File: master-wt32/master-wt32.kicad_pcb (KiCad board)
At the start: 2 copper layers, 64.6 x 72.4 mm, 24 parts, among them J1 Screw_Terminal_01x04, J2 Screw_Terminal_01x03, J3 Conn_01x06_Female, J4 Conn_01x06_Female, SW1 SW_DIP_x02, U1 MINI360, U2 PC817, U3 WT32-ETH0-Board, U4 MINI360

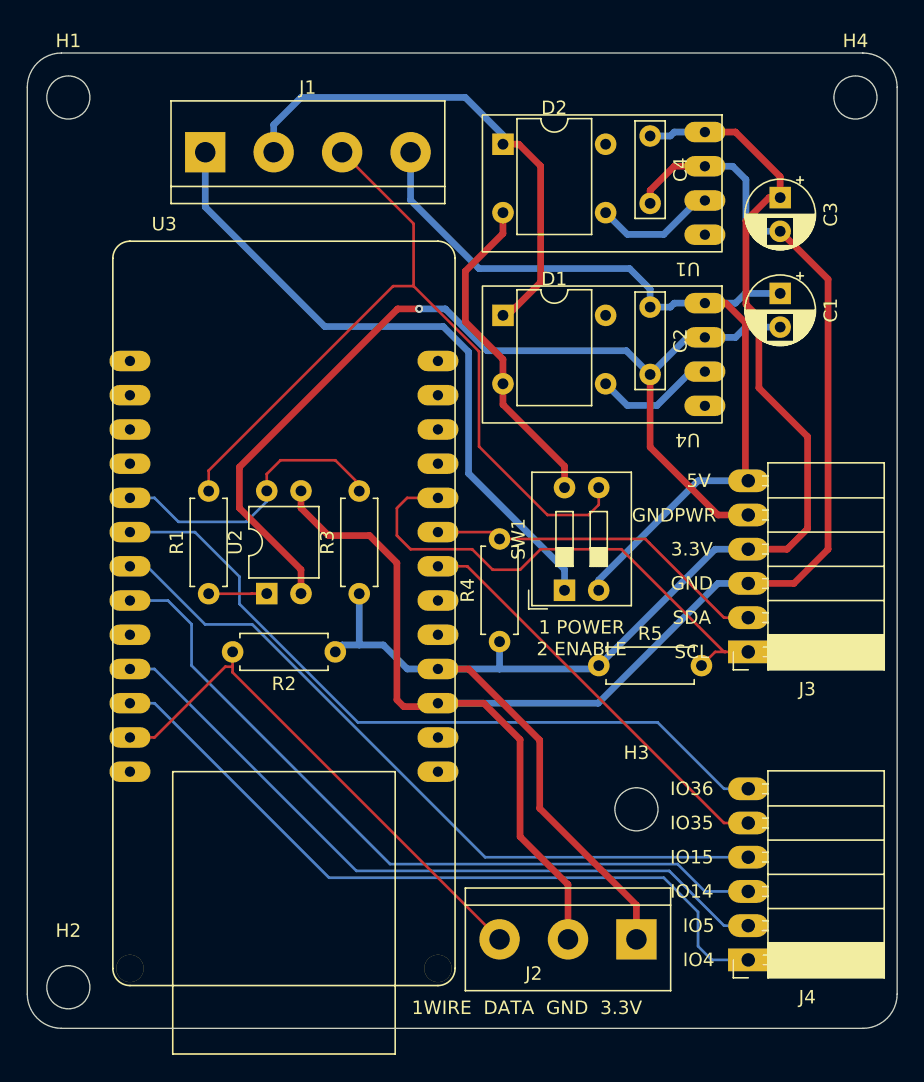
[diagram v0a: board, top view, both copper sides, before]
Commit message: route master-wt32
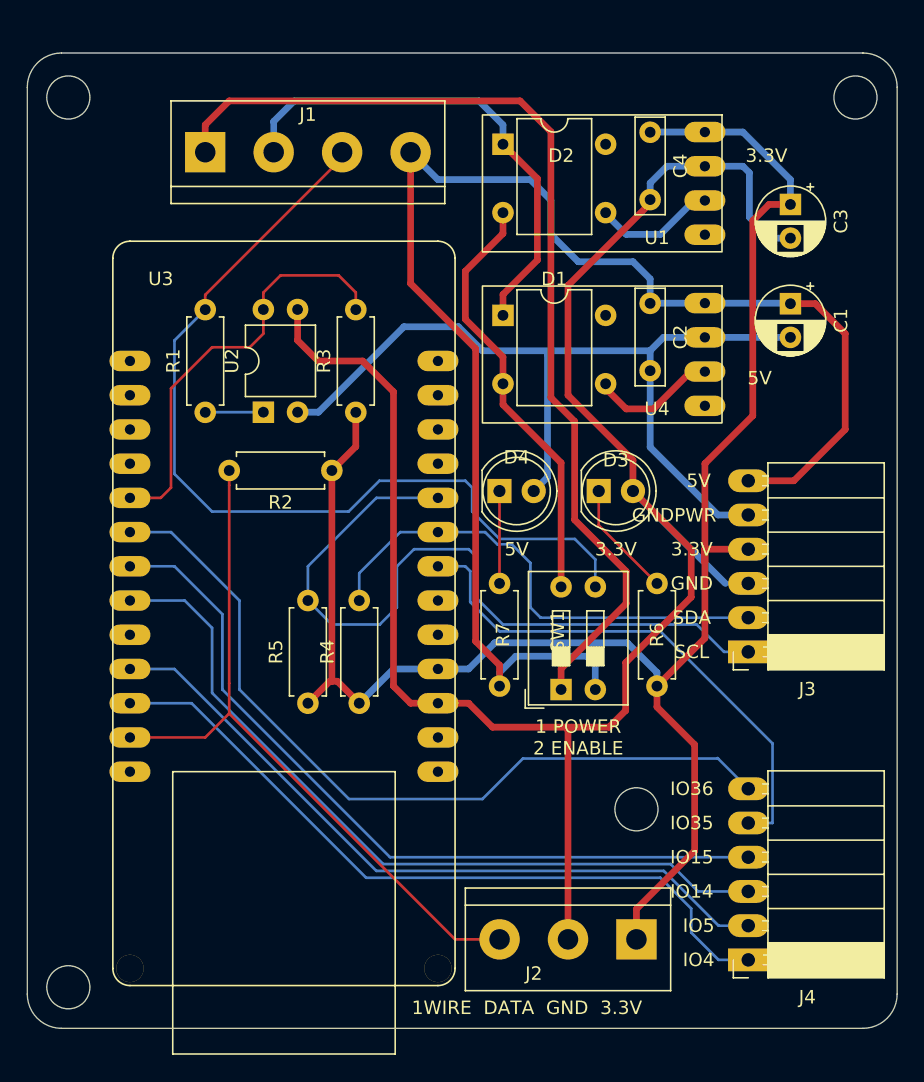
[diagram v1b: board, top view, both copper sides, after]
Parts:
- added D3: LED, LED_THT:LED_D5.0mm, F.Cu at (105.9, 87.1)
- added D4: LED, LED_THT:LED_D5.0mm, F.Cu at (98.5, 87.1)
- added R6: 330, Resistor_THT:R_Axial_DIN0207_L6.3mm_D2.5mm_P7.62mm_Horizontal, F.Cu at (110.2, 94.0)
- added R7: 680, Resistor_THT:R_Axial_DIN0207_L6.3mm_D2.5mm_P7.62mm_Horizontal, F.Cu at (98.6, 94.0)
- moved R5 21.8 mm to (84.3, 102.9), turned to 90 degrees
- moved R1 13.5 mm to (76.7, 81.3)
- moved R2 13.5 mm to (86.1, 85.6)
- moved R3 13.5 mm to (87.9, 81.3)
- moved U2 13.5 mm to (81.0, 81.3)
- moved R4 11.4 mm to (88.1, 102.9)
- moved SW1 7.37 mm to (103.1, 101.9)
- moved C1 1.08 mm to (120.1, 73.2)
- moved C3 0.92 mm to (120.1, 65.9)
- moved C2 0.28 mm to (109.7, 73.2)
- moved C4 0.28 mm to (109.7, 60.5)
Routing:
- net +5V: track 65.8 -> 109.4 mm
- net Net-(J1-Pad1): track 48.7 -> 75.1 mm
- net GND: track 121.0 -> 139.7 mm
- net SCL: track 38.5 -> 56.8 mm
- net +3V3: track 114.4 -> 132.2 mm
- net 1WIRE: track 39.3 -> 53.1 mm
- net SDA: track 25.7 -> 36.7 mm
- net ENABLE: track 22.1 -> 31.5 mm
- net Net-(D3-Pad1): track 0.00 -> 8.65 mm
- net GPIO35: track 30.9 -> 39.3 mm
- net IN+: track 24.6 -> 31.9 mm
- net Net-(D4-Pad1): track 0.00 -> 6.86 mm
- net ENABLE_IN: track 61.0 -> 67.9 mm
- net GNDPWR: track 74.5 -> 67.8 mm, vias 1 -> 0
- net GPIO36: track 55.0 -> 60.2 mm
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
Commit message: refactor master-wt32 pcb
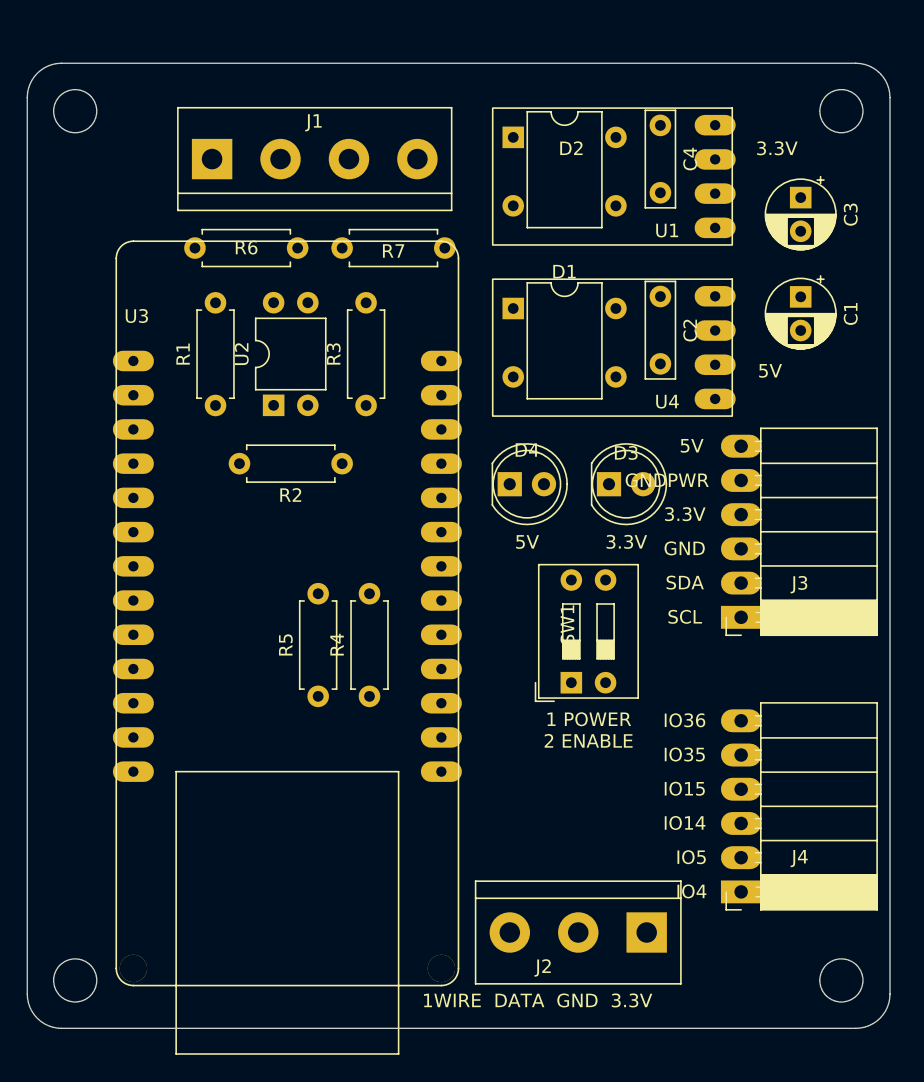
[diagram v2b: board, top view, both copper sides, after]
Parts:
- moved H2 86.7 mm to (123.9, 58.9)
- moved H4 65.5 mm to (123.9, 123.4)
- moved H3 43.5 mm to (67.1, 123.4)
- moved R6 36.5 mm to (83.6, 69.1), turned to 180 degrees
- moved R7 25.2 mm to (94.5, 69.1), turned to 180 degrees
- moved J4 5.07 mm to (116.5, 116.9)
- moved J3 2.62 mm to (116.5, 96.5)
- moved H1 1.14 mm to (67.1, 58.9)
- moved R4 0.92 mm to (88.9, 102.4)
- moved R5 0.92 mm to (85.1, 102.4)
- moved U4 0.92 mm to (106.9, 76.5)
- moved D2 0.92 mm to (99.6, 60.9)
- moved U1 0.92 mm to (106.9, 63.8)
- moved C2 0.92 mm to (110.5, 72.7)
- moved C3 0.92 mm to (120.9, 65.3)
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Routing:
- net GND: track 139.7 -> 0.00 mm
- net +3V3: track 132.2 -> 0.00 mm
- net +5V: track 109.4 -> 0.00 mm
- net Net-(J1-Pad1): track 75.1 -> 0.00 mm
- net ENABLE_IN: track 67.9 -> 0.00 mm
- net GNDPWR: track 67.8 -> 0.00 mm
- net GPIO36: track 60.2 -> 0.00 mm
- net GPIO15: track 58.1 -> 0.00 mm
- net GPIO14: track 57.7 -> 0.00 mm
- net SCL: track 56.8 -> 0.00 mm
- net GPIO4: track 54.8 -> 0.00 mm
- net GPIO5: track 53.8 -> 0.00 mm
- net 1WIRE: track 53.1 -> 0.00 mm
- net GPIO35: track 39.3 -> 0.00 mm
- net IN-: track 36.9 -> 0.00 mm
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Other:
- board size 64.6 x 72.4 mm -> 64 x 71.6 mm
